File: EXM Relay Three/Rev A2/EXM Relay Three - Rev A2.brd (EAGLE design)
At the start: 80 x 50 mm, 24 parts, among them J1 22-05-7048-04, J10 MSTBA3, J2 22-05-7048-04, J3 MSTBA3, J4 22-05-7048-04, J5 22-05-7048-04, J6 MSTBA3, J7 22-05-7048-04, J8 22-05-7048-04, J9 MSTBA2, K1 MY2, K2 MY2, K3 MY2, T1 EXMACHINA-LOGO-NAME

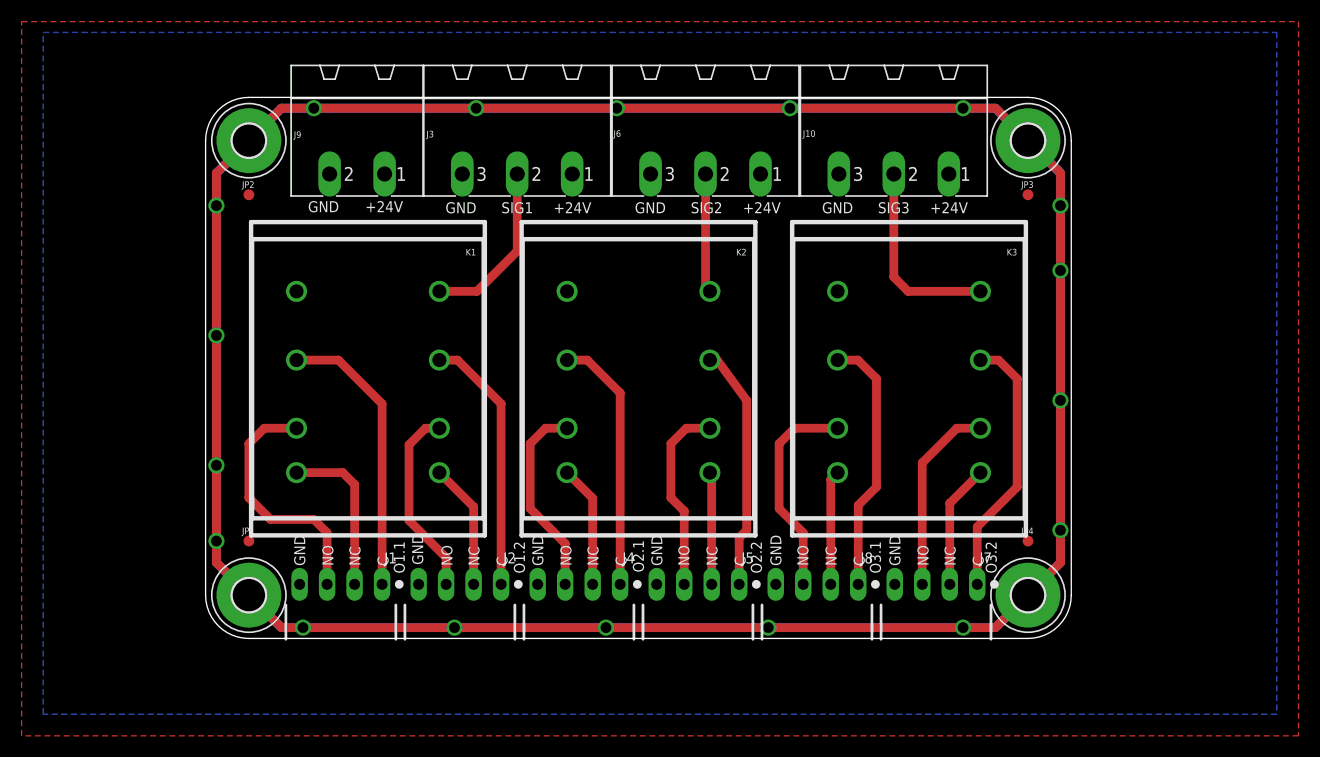
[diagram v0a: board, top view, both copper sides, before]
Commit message: Renumber part and updated BOM
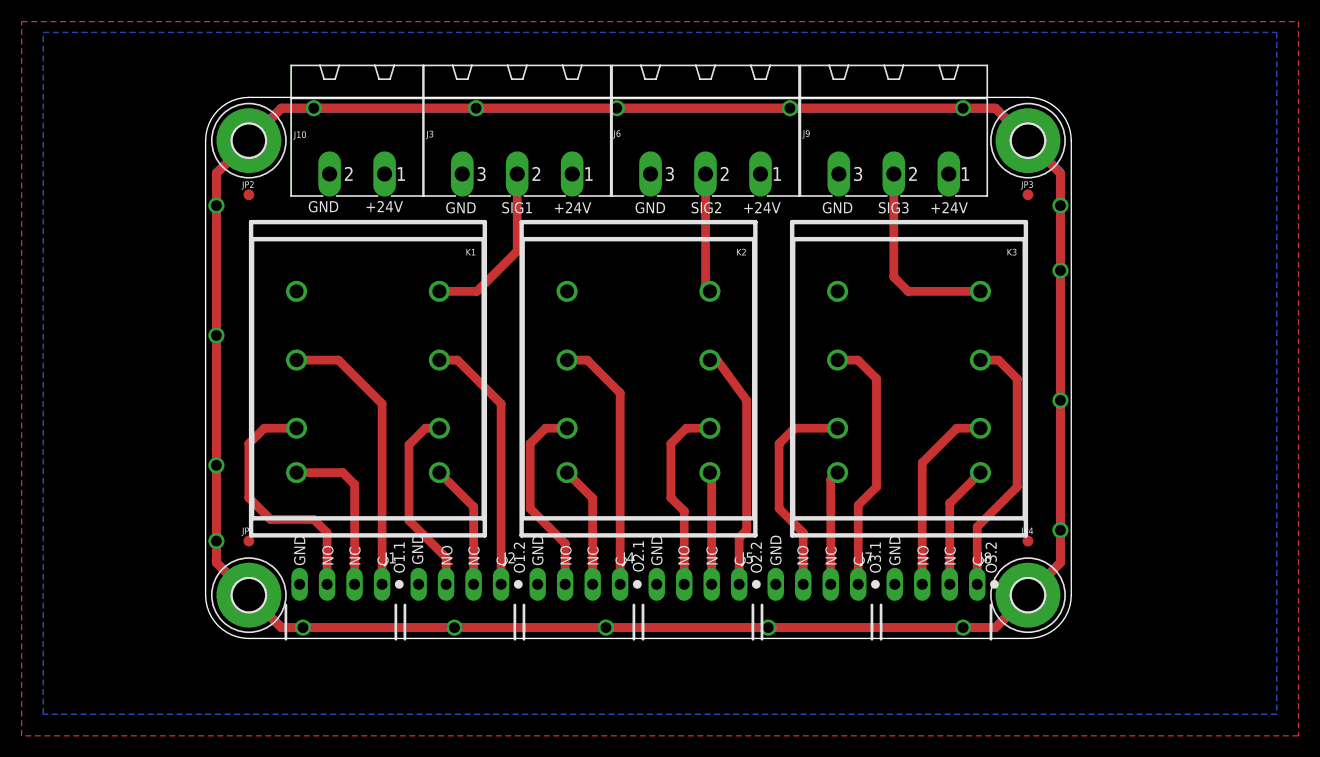
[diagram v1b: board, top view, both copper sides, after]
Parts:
- J10: value MSTBA3 -> MSTBA2; device con-phoenix-508:MSTBA3 -> con-phoenix-508:MSTBA2
- J9: value MSTBA2 -> MSTBA3; device con-phoenix-508:MSTBA2 -> con-phoenix-508:MSTBA3
- moved J10 49.6 mm to (14.0, 48.0)
- moved J9 49.6 mm to (63.6, 48.0)
- moved J7 11.0 mm to (56.5, 5.00)
- moved J8 11.0 mm to (67.5, 5.00)
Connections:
- net GND: now also J10.2, J9.3; no longer J10.3, J9.2
- net SIG3_1_C: now also J7.1; no longer J8.1
- net SIG3_1_NC: now also J7.2; no longer J8.2
- net SIG3_1_NO: now also J7.3; no longer J8.3
- net SIG3_2_C: now also J8.1; no longer J7.1
- net SIG3_2_NC: now also J8.2; no longer J7.2
- net SIG3_2_NO: now also J8.3; no longer J7.3
- net SIG_IN_3: now also J9.2; no longer J10.2
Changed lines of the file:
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@@
 <attribute name="MPN" value="PY08" x="40" y="24" size="1.778" layer="27" rot="R180" display="off"/>
 </element>
-<element name="J10" library="con-phoenix-508" package="MSTBA3" value="MSTBA3" x="63.6" y="48" smashed="yes" rot="R180">
+<element name="J9" library="con-phoenix-508" package="MSTBA3" value="MSTBA3" x="63.6" y="48" smashed="yes" rot="R180">
 <attribute name="MPN" value="1757255" x="63.6" y="-17" size="1.778" layer="27" rot="R180" display="off"/>
 <attribute name="MF" value="FARNELL" x="63.6" y="-17" size="1.778" layer="27" rot="R180" display="off"/>
@@
 <attribute name="MPN" value="PY08" x="65" y="24" size="1.778" layer="27" rot="R180" display="off"/>
 </element>
-<element name="J9" library="con-phoenix-508" package="MSTBA2" value="MSTBA2" x="14" y="48" smashed="yes" rot="R180">
+<element name="J10" library="con-phoenix-508" package="MSTBA2" value="MSTBA2" x="14" y="48" smashed="yes" rot="R180">
 <attribute name="MPN" value="1757242" x="14" y="48" size="1.778" layer="27" rot="R180" display="off"/>
 <attribute name="MF" value="FARNELL" x="14" y="48" size="1.778" layer="27" rot="R180" display="off"/>
@@
 <attribute name="OC_NEWARK" value="unknown" x="34.5" y="5" size="1.778" layer="27" display="off"/>
 </element>
-<element name="J7" library="con-molex" package="7395-04" value="22-05-7048-04" x="67.5" y="5">
+<element name="J8" library="con-molex" package="7395-04" value="22-05-7048-04" x="67.5" y="5">
 <attribute name="MF" value="" x="67.5" y="5" size="1.778" layer="27" display="off"/>
 <attribute name="MPN" value="" x="67.5" y="5" size="1.778" layer="27" display="off"/>
@@
 <attribute name="OC_NEWARK" value="unknown" x="67.5" y="5" size="1.778" layer="27" display="off"/>
 </element>
-<element name="J8" library="con-molex" package="7395-04" value="22-05-7048-04" x="56.5" y="5">
+<element name="J7" library="con-molex" package="7395-04" value="22-05-7048-04" x="56.5" y="5">
 <attribute name="MF" value="" x="56.5" y="5" size="1.778" layer="27" display="off"/>
 <attribute name="MPN" value="" x="56.5" y="5" size="1.778" layer="27" display="off"/>
@@
 </polygon>
 <contactref element="J6" pad="1"/>
+<contactref element="J9" pad="1"/>
 <contactref element="J10" pad="1"/>
-<contactref element="J9" pad="1"/>
 </signal>
 <signal name="GND">
@@
 <contactref element="J6" pad="3"/>
 <contactref element="K2" pad="13"/>
-<contactref element="J10" pad="3"/>
+<contactref element="J9" pad="3"/>
 <contactref element="K3" pad="13"/>
-<contactref element="J9" pad="2"/>
+<contactref element="J10" pad="2"/>
 <contactref element="J2" pad="4"/>
 <contactref element="J1" pad="4"/>
 <contactref element="J5" pad="4"/>
 <contactref element="J4" pad="4"/>
+<contactref element="J8" pad="4"/>
 <contactref element="J7" pad="4"/>
-<contactref element="J8" pad="4"/>
 </signal>
 <signal name="SIG_IN_2">
@@
 <signal name="SIG3_2_NC">
 <contactref element="K3" pad="4"/>
-<contactref element="J7" pad="2"/>
+<contactref element="J8" pad="2"/>
 <wire x1="68.77" y1="5" x2="68.77" y2="12.49" width="0.8128" layer="1"/>
 <wire x1="68.77" y1="12.49" x2="71.605" y2="15.325" width="0.8128" layer="1"/>
@@
 <contactref element="K3" pad="8"/>
 <wire x1="69.425" y1="19.425" x2="71.605" y2="19.425" width="0.8128" layer="1"/>
-<contactref element="J7" pad="3"/>
+<contactref element="J8" pad="3"/>
 <wire x1="66.23" y1="5" x2="66.23" y2="16.23" width="0.8128" layer="1"/>
 <wire x1="66.23" y1="16.23" x2="69.425" y2="19.425" width="0.8128" layer="1"/>
@@
 <signal name="SIG3_1_NC">
 <contactref element="K3" pad="1"/>
-<contactref element="J8" pad="2"/>
+<contactref element="J7" pad="2"/>
 <wire x1="57.77" y1="5" x2="57.77" y2="14.69" width="0.8128" layer="1"/>
 <wire x1="57.77" y1="14.69" x2="58.405" y2="15.325" width="0.8128" layer="1"/>
@@
 <wire x1="53" y1="18" x2="54.425" y2="19.425" width="0.8128" layer="1"/>
 <wire x1="54.425" y1="19.425" x2="58.405" y2="19.425" width="0.8128" layer="1"/>
-<contactref element="J8" pad="3"/>
+<contactref element="J7" pad="3"/>
 <wire x1="53" y1="12" x2="55.23" y2="9.77" width="0.8128" layer="1"/>
 <wire x1="55.23" y1="9.77" x2="55.23" y2="5" width="0.8128" layer="1"/>
 </signal>
 <signal name="SIG_IN_3">
-<contactref element="J10" pad="2"/>
+<contactref element="J9" pad="2"/>
 <contactref element="K3" pad="14"/>
 <wire x1="71.605" y1="32.075" x2="64.925" y2="32.075" width="0.8128" layer="1"/>
@@
 <signal name="SIG3_2_C">
 <contactref element="K3" pad="12"/>
-<contactref element="J7" pad="1"/>
+<contactref element="J8" pad="1"/>
 <wire x1="71.31" y1="5" x2="71.31" y2="10.31" width="0.8128" layer="1"/>
 <wire x1="71.31" y1="10.31" x2="75" y2="14" width="0.8128" layer="1"/>
@@
 <signal name="SIG3_1_C">
 <contactref element="K3" pad="9"/>
-<contactref element="J8" pad="1"/>
+<contactref element="J7" pad="1"/>
 <wire x1="60.31" y1="5" x2="60.31" y2="12.31" width="0.8128" layer="1"/>
 <wire x1="60.31" y1="12.31" x2="62" y2="14" width="0.8128" layer="1"/>
